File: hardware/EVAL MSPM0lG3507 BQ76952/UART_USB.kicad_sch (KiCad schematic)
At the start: 9 parts, among them J16 USB_B_Micro, U1 ISO7721D, U12 FT230XS, U4 ISO7721D, U8 L78L05_SOT89

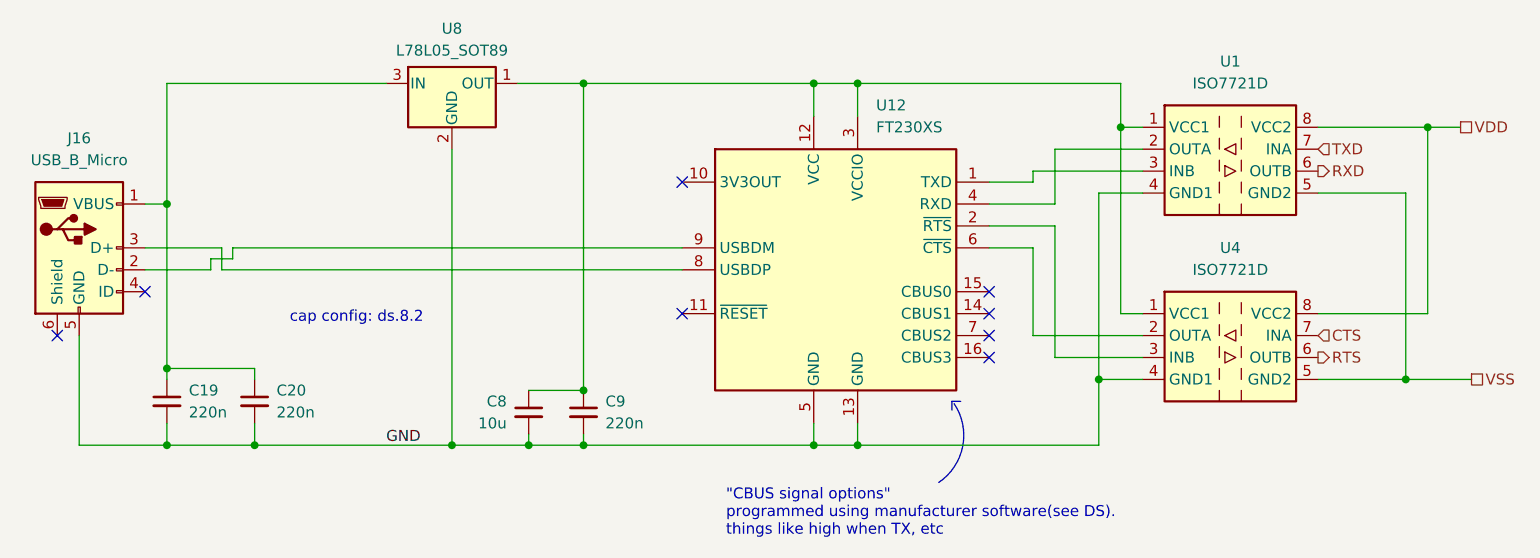
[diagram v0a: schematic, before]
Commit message: ac;lkacnl;
acea;kca
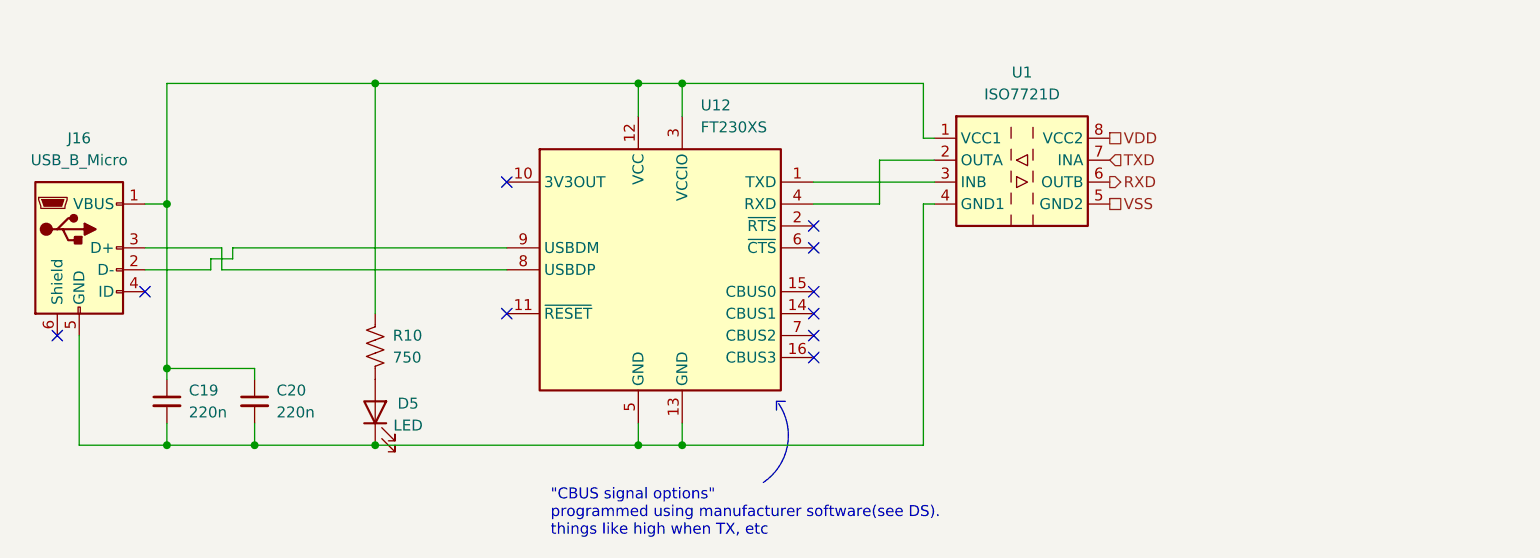
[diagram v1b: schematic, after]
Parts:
- removed C8: 10u, Capacitor_SMD:C_1206_3216Metric_Pad1.33x1.80mm_HandSolder, symbol Device:C_Small
- removed C9: 220n, Capacitor_SMD:C_1206_3216Metric_Pad1.33x1.80mm_HandSolder, symbol Device:C_Small
- removed U4: ISO7721D, Package_SO:SOIC-8_3.9x4.9mm_P1.27mm, symbol Isolator:ISO7721D
- removed U8: L78L05_SOT89, Package_TO_SOT_SMD:SOT-89-3, symbol Regulator_Linear:L78L05_SOT89
- added D5: LED, LED_SMD:LED_0603_1608Metric, symbol Device:LED
- added R10: 750, Resistor_SMD:R_1206_3216Metric_Pad1.30x1.75mm_HandSolder, symbol Device:R_US
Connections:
- net at U1.1 (VCC1), U12.12 (VCC), U12.3 (VCCIO): now also C19.1, C20.1, J16.1 (VBUS), R10.1
- net GND: no longer names the net of C19.2, C20.2, J16.5 (GND), U1.4 (GND1), U12.13 (GND), U12.5 (GND)
- net GND: now also D5.1 (K)
- new net: D5.2 (A), R10.2
- no-connect marks 8 -> 10
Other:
- note removed: "cap config: ds.8.2"
- moved on the sheet: U1, U12
